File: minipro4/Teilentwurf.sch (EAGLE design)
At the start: 89 parts, among them IC1 MEGA8-P, IC2 FT232RL_ADAPTER, IC3 78L08Z, IC4 4051N, IC5 TL082P, IC6 4051N, IC7 TL082P, J1 HOHLSTECKER, Q2 BS170, Q3 BS170, Q4 BS170, Q6 IRF4905, X1 , X2 CON_COAX

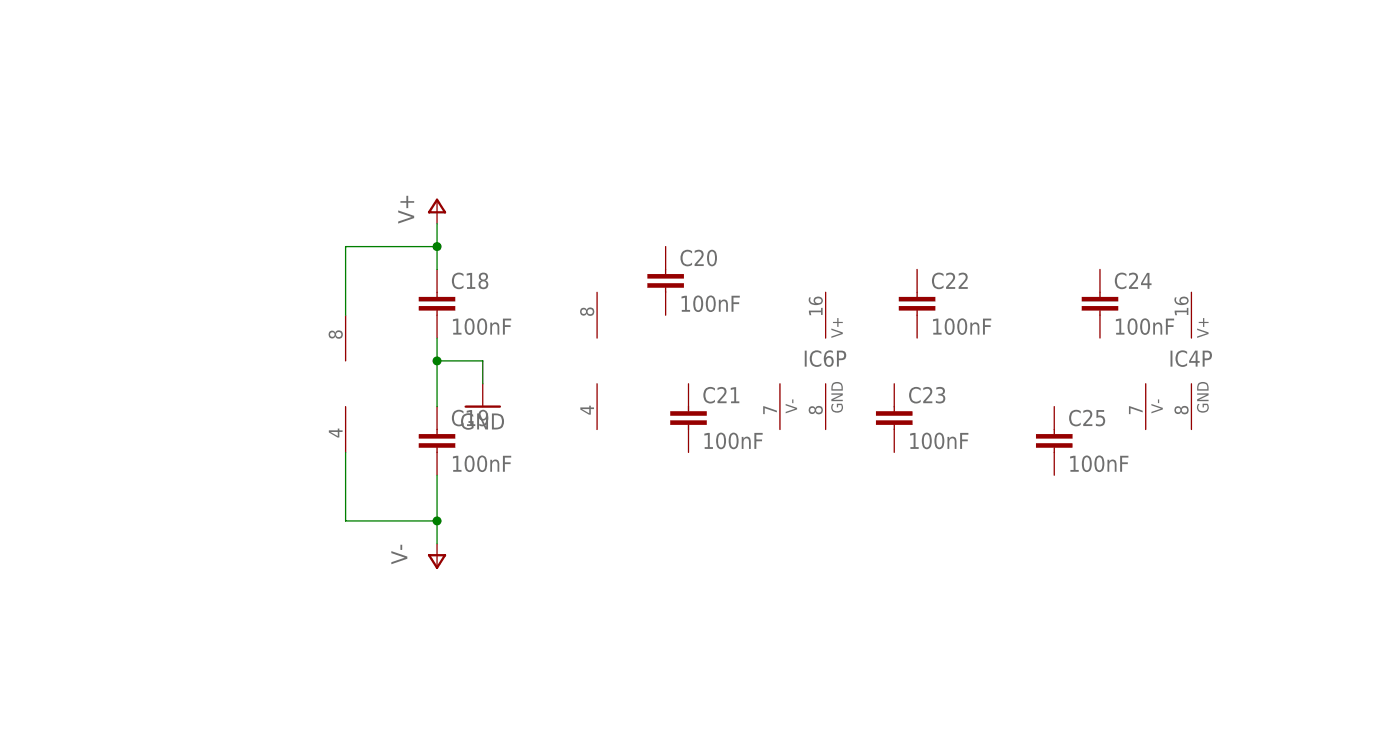
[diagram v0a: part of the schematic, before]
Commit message: eagle iteration
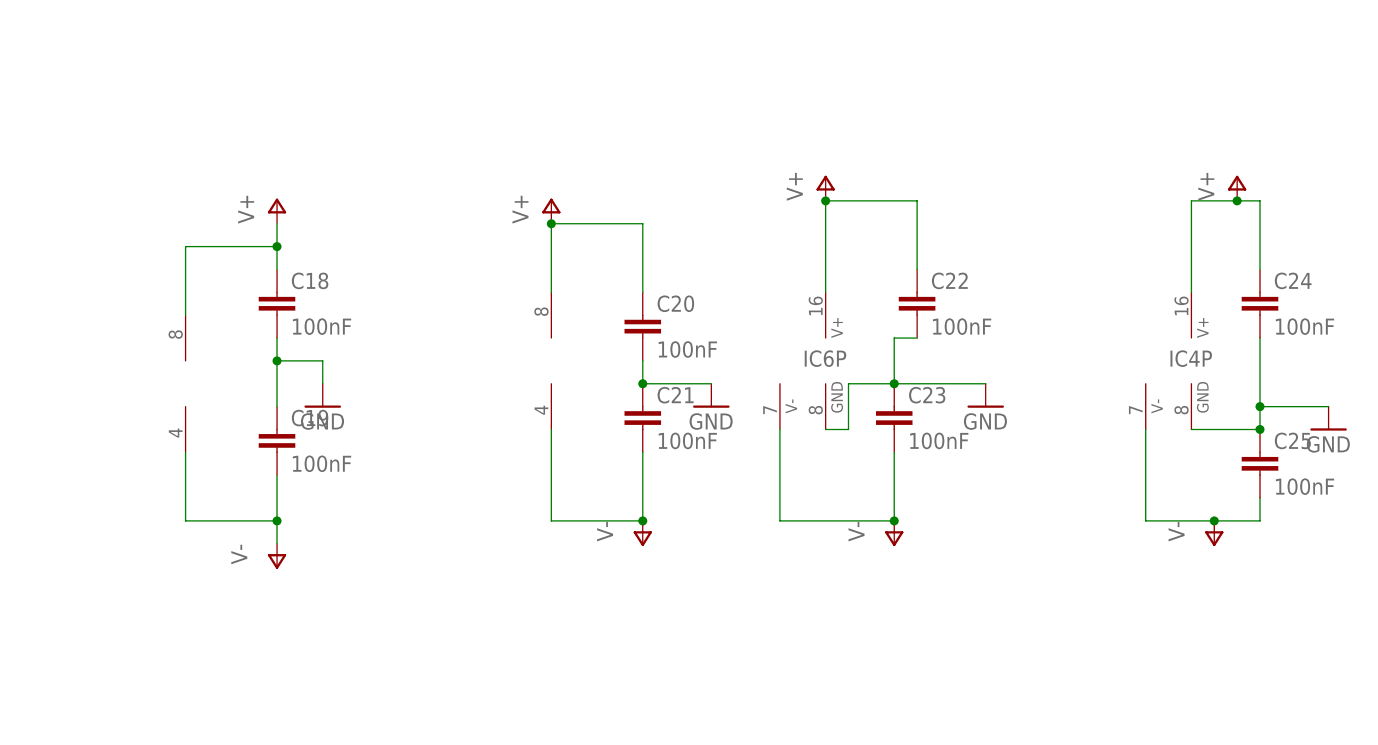
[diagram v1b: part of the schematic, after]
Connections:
- net GND: now also C20.2, C21.1, C22.2, C23.1, C24.2, C25.1, IC4P.GND, IC6P.GND
- net V+: now also C20.1, C22.1, C24.1, IC4P.V+, IC6P.V+, IC7P.V+
- net V-: now also C21.2, C23.2, C25.2, IC4P.V-, IC6P.V-, IC7P.V-
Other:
- moved on the sheet: C18, C19, C20, C21, C24, C25
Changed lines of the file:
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@@
 <part name="P+5" library="03_device-library" deviceset="V+" device=""/>
 <part name="P-3" library="03_device-library" deviceset="V-" device=""/>
+<part name="P+8" library="03_device-library" deviceset="V+" device=""/>
+<part name="P+9" library="03_device-library" deviceset="V+" device=""/>
+<part name="P+12" library="03_device-library" deviceset="V+" device=""/>
+<part name="P-4" library="03_device-library" deviceset="V-" device=""/>
+<part name="P-5" library="03_device-library" deviceset="V-" device=""/>
+<part name="P-6" library="03_device-library" deviceset="V-" device=""/>
+<part name="GND19" library="03_device-library" deviceset="GND" device=""/>
+<part name="GND20" library="03_device-library" deviceset="GND" device=""/>
+<part name="GND21" library="03_device-library" deviceset="GND" device=""/>
 </parts>
 <sheets>
@@
 <instance part="C17" gate="G$1" x="355.6" y="-35.56"/>
 <instance part="GND17" gate="1" x="355.6" y="-48.26"/>
-<instance part="C18" gate="G$1" x="304.8" y="73.66"/>
-<instance part="C19" gate="G$1" x="304.8" y="58.42"/>
-<instance part="C20" gate="G$1" x="330.2" y="76.2"/>
-<instance part="C21" gate="G$1" x="332.74" y="60.96"/>
+<instance part="C18" gate="G$1" x="287.02" y="73.66"/>
+<instance part="C19" gate="G$1" x="287.02" y="58.42"/>
+<instance part="C20" gate="G$1" x="327.66" y="71.12"/>
+<instance part="C21" gate="G$1" x="327.66" y="60.96"/>
 <instance part="C22" gate="G$1" x="358.14" y="73.66"/>
 <instance part="C23" gate="G$1" x="355.6" y="60.96"/>
-<instance part="C24" gate="G$1" x="378.46" y="73.66"/>
-<instance part="C25" gate="G$1" x="373.38" y="58.42"/>
-<instance part="IC5" gate="P" x="294.64" y="63.5"/>
-<instance part="IC7" gate="P" x="322.58" y="66.04"/>
+<instance part="C24" gate="G$1" x="396.24" y="73.66"/>
+<instance part="C25" gate="G$1" x="396.24" y="55.88"/>
+<instance part="IC5" gate="P" x="276.86" y="63.5"/>
+<instance part="IC7" gate="P" x="317.5" y="66.04"/>
 <instance part="IC6" gate="P" x="347.98" y="66.04"/>
 <instance part="IC4" gate="P" x="388.62" y="66.04"/>
-<instance part="GND18" gate="1" x="309.88" y="60.96"/>
-<instance part="P+5" gate="1" x="304.8" y="83.82"/>
-<instance part="P-3" gate="1" x="304.8" y="43.18"/>
+<instance part="GND18" gate="1" x="292.1" y="60.96"/>
+<instance part="P+5" gate="1" x="287.02" y="83.82"/>
+<instance part="P-3" gate="1" x="287.02" y="43.18"/>
+<instance part="P+8" gate="1" x="317.5" y="83.82"/>
+<instance part="P+9" gate="1" x="347.98" y="86.36"/>
+<instance part="P+12" gate="1" x="393.7" y="86.36"/>
+<instance part="P-4" gate="1" x="327.66" y="45.72"/>
+<instance part="P-5" gate="1" x="355.6" y="45.72"/>
+<instance part="P-6" gate="1" x="391.16" y="45.72"/>
+<instance part="GND19" gate="1" x="335.28" y="60.96"/>
+<instance part="GND20" gate="1" x="365.76" y="60.96"/>
+<instance part="GND21" gate="1" x="403.86" y="58.42"/>
 </instances>
 <busses>
@@
 <pinref part="C18" gate="G$1" pin="2"/>
 <pinref part="C19" gate="G$1" pin="1"/>
-<wire x1="304.8" y1="68.58" x2="304.8" y2="66.04" width="0.1524" layer="91"/>
-<wire x1="304.8" y1="66.04" x2="304.8" y2="60.96" width="0.1524" layer="91"/>
-<wire x1="304.8" y1="66.04" x2="309.88" y2="66.04" width="0.1524" layer="91"/>
-<wire x1="309.88" y1="66.04" x2="309.88" y2="63.5" width="0.1524" layer="91"/>
-<junction x="304.8" y="66.04"/>
+<wire x1="287.02" y1="68.58" x2="287.02" y2="66.04" width="0.1524" layer="91"/>
+<wire x1="287.02" y1="66.04" x2="287.02" y2="60.96" width="0.1524" layer="91"/>
+<wire x1="287.02" y1="66.04" x2="292.1" y2="66.04" width="0.1524" layer="91"/>
+<wire x1="292.1" y1="66.04" x2="292.1" y2="63.5" width="0.1524" layer="91"/>
+<junction x="287.02" y="66.04"/>
 <pinref part="GND18" gate="1" pin="GND"/>
+</segment>
+<segment>
+<pinref part="C20" gate="G$1" pin="2"/>
+<pinref part="C21" gate="G$1" pin="1"/>
+<wire x1="327.66" y1="66.04" x2="327.66" y2="63.5" width="0.1524" layer="91"/>
+<pinref part="GND19" gate="1" pin="GND"/>
+<wire x1="335.28" y1="63.5" x2="327.66" y2="63.5" width="0.1524" layer="91"/>
+<junction x="327.66" y="63.5"/>
+</segment>
+<segment>
+<pinref part="IC6" gate="P" pin="GND"/>
+<wire x1="347.98" y1="58.42" x2="350.52" y2="58.42" width="0.1524" layer="91"/>
+<wire x1="350.52" y1="58.42" x2="350.52" y2="63.5" width="0.1524" layer="91"/>
+<pinref part="C23" gate="G$1" pin="1"/>
+<wire x1="350.52" y1="63.5" x2="355.6" y2="63.5" width="0.1524" layer="91"/>
+<pinref part="C22" gate="G$1" pin="2"/>
+<wire x1="358.14" y1="68.58" x2="355.6" y2="68.58" width="0.1524" layer="91"/>
+<wire x1="355.6" y1="68.58" x2="355.6" y2="63.5" width="0.1524" layer="91"/>
+<junction x="355.6" y="63.5"/>
+<pinref part="GND20" gate="1" pin="GND"/>
+<wire x1="365.76" y1="63.5" x2="355.6" y2="63.5" width="0.1524" layer="91"/>
+</segment>
+<segment>
+<pinref part="C25" gate="G$1" pin="1"/>
+<pinref part="C24" gate="G$1" pin="2"/>
+<wire x1="396.24" y1="58.42" x2="396.24" y2="60.96" width="0.1524" layer="91"/>
+<pinref part="IC4" gate="P" pin="GND"/>
+<wire x1="396.24" y1="60.96" x2="396.24" y2="68.58" width="0.1524" layer="91"/>
+<wire x1="388.62" y1="58.42" x2="396.24" y2="58.42" width="0.1524" layer="91"/>
+<junction x="396.24" y="58.42"/>
+<pinref part="GND21" gate="1" pin="GND"/>
+<wire x1="403.86" y1="60.96" x2="396.24" y2="60.96" width="0.1524" layer="91"/>
+<junction x="396.24" y="60.96"/>
 </segment>
 </net>
@@
 <segment>
 <pinref part="C18" gate="G$1" pin="1"/>
-<wire x1="304.8" y1="76.2" x2="304.8" y2="78.74" width="0.1524" layer="91"/>
+<wire x1="287.02" y1="76.2" x2="287.02" y2="78.74" width="0.1524" layer="91"/>
 <pinref part="IC5" gate="P" pin="V+"/>
-<wire x1="304.8" y1="78.74" x2="294.64" y2="78.74" width="0.1524" layer="91"/>
-<wire x1="294.64" y1="78.74" x2="294.64" y2="71.12" width="0.1524" layer="91"/>
-<wire x1="304.8" y1="78.74" x2="304.8" y2="81.28" width="0.1524" layer="91"/>
-<junction x="304.8" y="78.74"/>
+<wire x1="287.02" y1="78.74" x2="276.86" y2="78.74" width="0.1524" layer="91"/>
+<wire x1="276.86" y1="78.74" x2="276.86" y2="71.12" width="0.1524" layer="91"/>
+<wire x1="287.02" y1="78.74" x2="287.02" y2="81.28" width="0.1524" layer="91"/>
+<junction x="287.02" y="78.74"/>
 <pinref part="P+5" gate="1" pin="V+"/>
+</segment>
+<segment>
+<pinref part="IC7" gate="P" pin="V+"/>
+<wire x1="317.5" y1="73.66" x2="317.5" y2="81.28" width="0.1524" layer="91"/>
+<wire x1="317.5" y1="81.28" x2="327.66" y2="81.28" width="0.1524" layer="91"/>
+<pinref part="C20" gate="G$1" pin="1"/>
+<wire x1="327.66" y1="81.28" x2="327.66" y2="73.66" width="0.1524" layer="91"/>
+<pinref part="P+8" gate="1" pin="V+"/>
+<junction x="317.5" y="81.28"/>
+</segment>
+<segment>
+<pinref part="C22" gate="G$1" pin="1"/>
+<wire x1="358.14" y1="76.2" x2="358.14" y2="83.82" width="0.1524" layer="91"/>
+<pinref part="IC6" gate="P" pin="V+"/>
+<wire x1="358.14" y1="83.82" x2="347.98" y2="83.82" width="0.1524" layer="91"/>
+<wire x1="347.98" y1="83.82" x2="347.98" y2="73.66" width="0.1524" layer="91"/>
+<pinref part="P+9" gate="1" pin="V+"/>
+<junction x="347.98" y="83.82"/>
+</segment>
+<segment>
+<pinref part="C24" gate="G$1" pin="1"/>
+<wire x1="396.24" y1="76.2" x2="396.24" y2="83.82" width="0.1524" layer="91"/>
+<pinref part="IC4" gate="P" pin="V+"/>
+<wire x1="396.24" y1="83.82" x2="393.7" y2="83.82" width="0.1524" layer="91"/>
+<wire x1="393.7" y1="83.82" x2="388.62" y2="83.82" width="0.1524" layer="91"/>
+<wire x1="388.62" y1="83.82" x2="388.62" y2="73.66" width="0.1524" layer="91"/>
+<pinref part="P+12" gate="1" pin="V+"/>
+<junction x="393.7" y="83.82"/>
 </segment>
 </net>
@@
 <segment>
 <pinref part="IC5" gate="P" pin="V-"/>
-<wire x1="294.64" y1="55.88" x2="294.64" y2="48.26" width="0.1524" layer="91"/>
+<wire x1="276.86" y1="55.88" x2="276.86" y2="48.26" width="0.1524" layer="91"/>
 <pinref part="C19" gate="G$1" pin="2"/>
-<wire x1="294.64" y1="48.26" x2="304.8" y2="48.26" width="0.1524" layer="91"/>
-<wire x1="304.8" y1="48.26" x2="304.8" y2="53.34" width="0.1524" layer="91"/>
-<wire x1="304.8" y1="48.26" x2="304.8" y2="45.72" width="0.1524" layer="91"/>
-<junction x="304.8" y="48.26"/>
+<wire x1="276.86" y1="48.26" x2="287.02" y2="48.26" width="0.1524" layer="91"/>
+<wire x1="287.02" y1="48.26" x2="287.02" y2="53.34" width="0.1524" layer="91"/>
+<wire x1="287.02" y1="48.26" x2="287.02" y2="45.72" width="0.1524" layer="91"/>
+<junction x="287.02" y="48.26"/>
 <pinref part="P-3" gate="1" pin="V-"/>
 </segment>
+<segment>
+<pinref part="C21" gate="G$1" pin="2"/>
+<wire x1="327.66" y1="55.88" x2="327.66" y2="48.26" width="0.1524" layer="91"/>
+<pinref part="IC7" gate="P" pin="V-"/>
+<wire x1="327.66" y1="48.26" x2="317.5" y2="48.26" width="0.1524" layer="91"/>
+<wire x1="317.5" y1="48.26" x2="317.5" y2="58.42" width="0.1524" layer="91"/>
+<pinref part="P-4" gate="1" pin="V-"/>
+<junction x="327.66" y="48.26"/>
+</segment>
+<segment>
+<pinref part="IC6" gate="P" pin="V-"/>
+<wire x1="342.9" y1="58.42" x2="342.9" y2="48.26" width="0.1524" layer="91"/>
+<pinref part="C23" gate="G$1" pin="2"/>
+<wire x1="342.9" y1="48.26" x2="355.6" y2="48.26" width="0.1524" layer="91"/>
+<wire x1="355.6" y1="48.26" x2="355.6" y2="55.88" width="0.1524" layer="91"/>
+<pinref part="P-5" gate="1" pin="V-"/>
+<junction x="355.6" y="48.26"/>
+</segment>
+<segment>
+<pinref part="IC4" gate="P" pin="V-"/>
+<wire x1="383.54" y1="58.42" x2="383.54" y2="48.26" width="0.1524" layer="91"/>
+<pinref part="C25" gate="G$1" pin="2"/>
+<wire x1="383.54" y1="48.26" x2="391.16" y2="48.26" width="0.1524" layer="91"/>
+<wire x1="391.16" y1="48.26" x2="396.24" y2="48.26" width="0.1524" layer="91"/>
+<wire x1="396.24" y1="48.26" x2="396.24" y2="50.8" width="0.1524" layer="91"/>
+<pinref part="P-6" gate="1" pin="V-"/>
+<junction x="391.16" y="48.26"/>
+</segment>
 </net>
